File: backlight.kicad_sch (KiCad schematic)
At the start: 56 parts

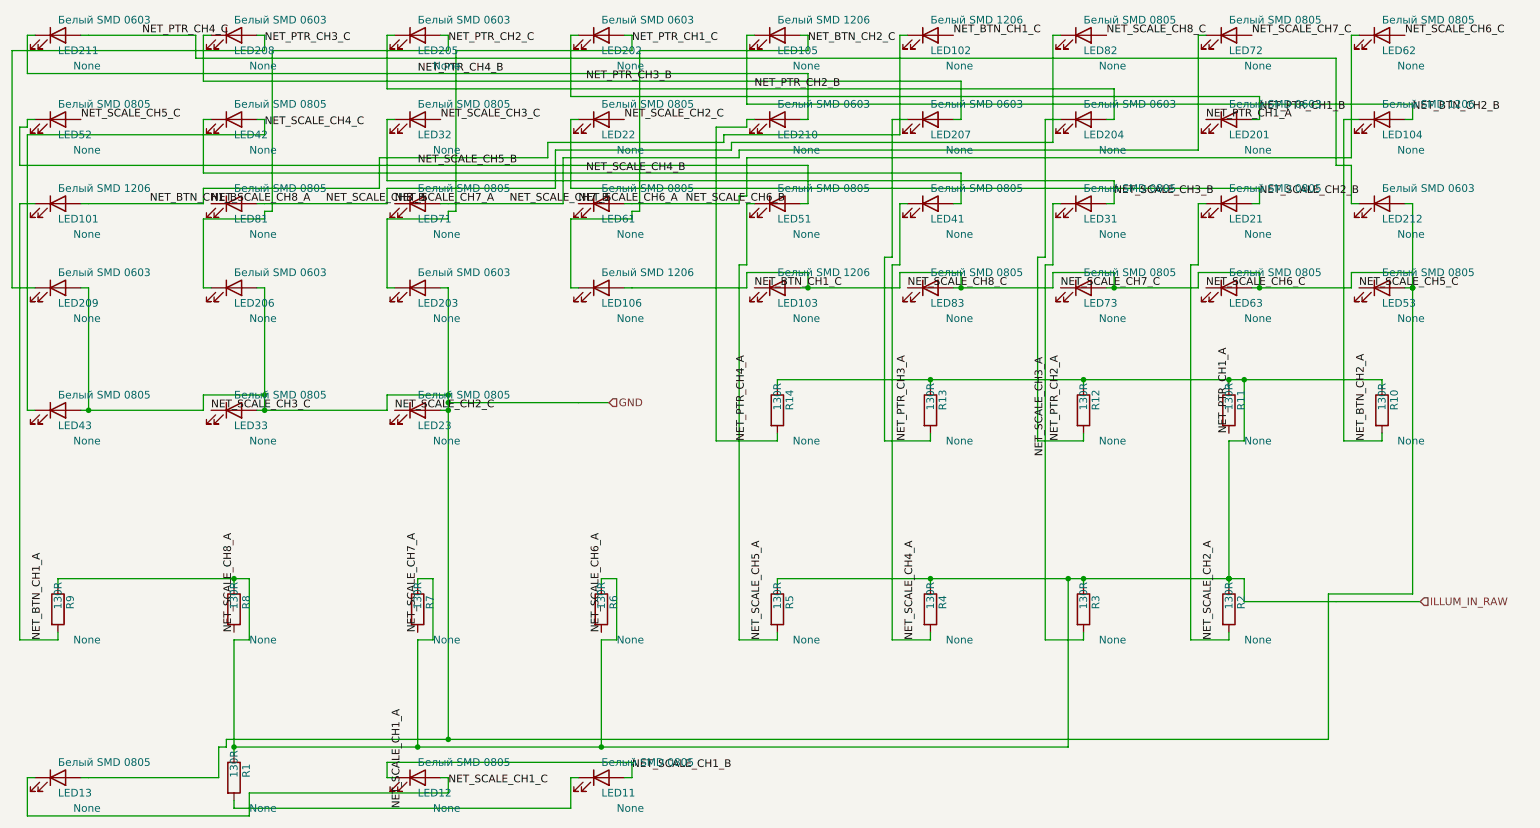
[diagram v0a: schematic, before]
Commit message: all unit test pass
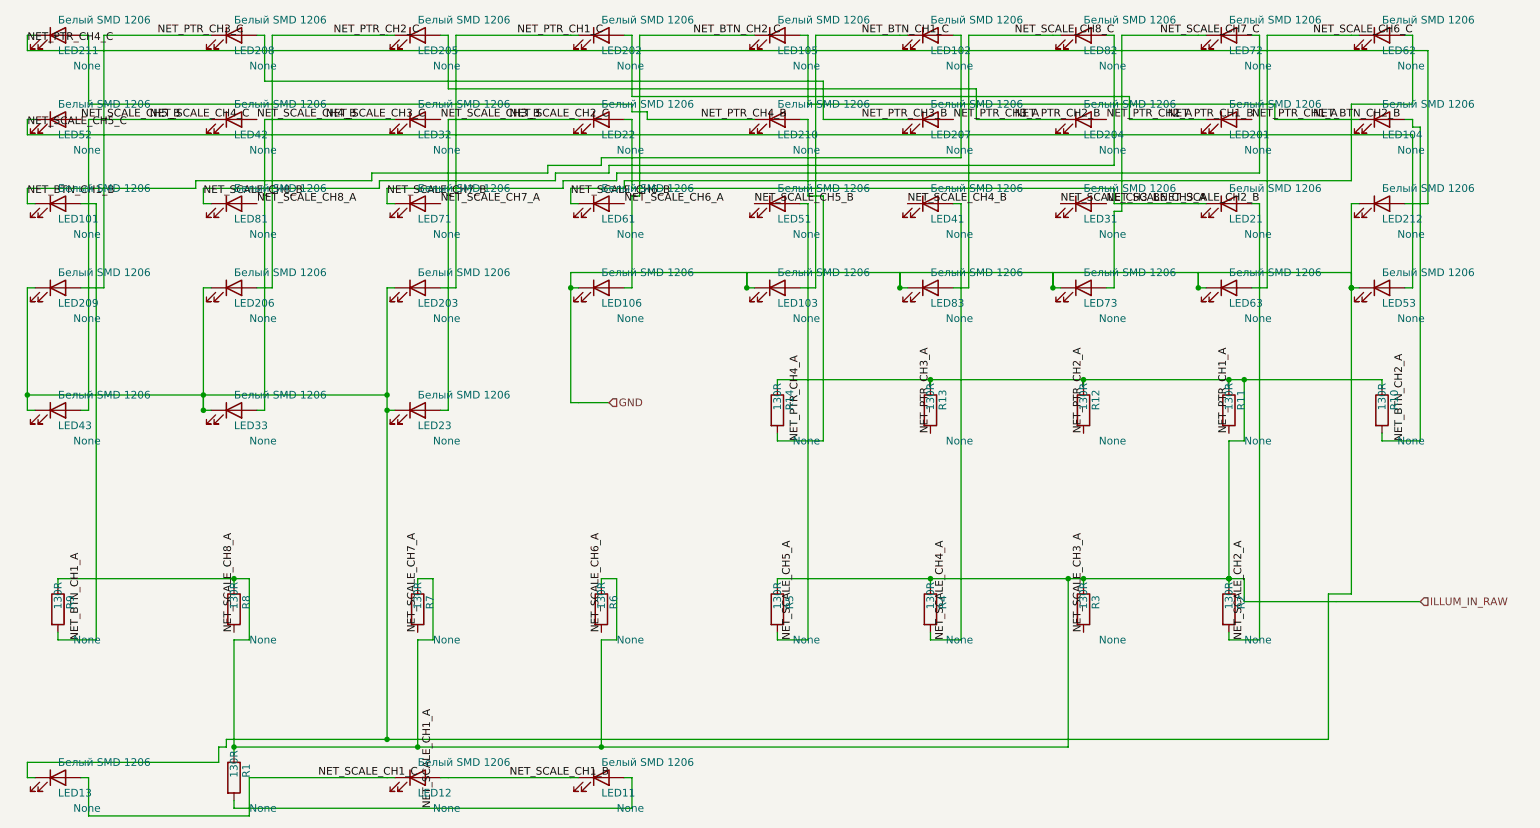
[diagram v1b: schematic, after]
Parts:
- LED11, LED12, LED13, LED21, LED22, LED23, LED31, LED32, LED33, LED41, LED42, LED43, LED51, LED52, LED53, LED61, LED62, LED63, LED71, LED72, LED73, LED81, LED82, LED83: value Белый SMD 0805 -> Белый SMD 1206
- LED201, LED202, LED203, LED204, LED205, LED206, LED207, LED208, LED209, LED210, LED211, LED212: value Белый SMD 0603 -> Белый SMD 1206
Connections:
- net GND: now also LED103.1 (K), LED106.1 (K), LED13.1 (K), LED203.1 (K), LED206.1 (K), LED209.1 (K), LED212.1 (K), LED23.1 (K), LED33.1 (K), LED43.1 (K), LED53.1 (K), LED63.1 (K), LED73.1 (K), LED83.1 (K); no longer LED103.2 (A), LED106.2 (A), LED13.2 (A), LED203.2 (A), LED206.2 (A), LED209.2 (A), LED212.2 (A), LED23.2 (A), LED33.2 (A), LED43.2 (A), LED53.2 (A), LED63.2 (A), LED73.2 (A), LED83.2 (A)
- net NET_BTN_CH1_A: now also LED101.2 (A); no longer LED101.1 (K)
- net NET_BTN_CH1_B: now also LED101.1 (K), LED102.2 (A); no longer LED101.2 (A), LED102.1 (K)
- net NET_BTN_CH1_C: now also LED102.1 (K), LED103.2 (A); no longer LED102.2 (A), LED103.1 (K)
- net NET_BTN_CH2_A: now also LED104.2 (A); no longer LED104.1 (K)
- net NET_BTN_CH2_B: now also LED104.1 (K), LED105.2 (A); no longer LED104.2 (A), LED105.1 (K)
- net NET_BTN_CH2_C: now also LED105.1 (K), LED106.2 (A); no longer LED105.2 (A), LED106.1 (K)
- net NET_PTR_CH1_A: now also LED201.2 (A); no longer LED201.1 (K)
- net NET_PTR_CH1_B: now also LED201.1 (K), LED202.2 (A); no longer LED201.2 (A), LED202.1 (K)
- net NET_PTR_CH1_C: now also LED202.1 (K), LED203.2 (A); no longer LED202.2 (A), LED203.1 (K)
- net NET_PTR_CH2_A: now also LED204.2 (A); no longer LED204.1 (K)
- net NET_PTR_CH2_B: now also LED204.1 (K), LED205.2 (A); no longer LED204.2 (A), LED205.1 (K)
- net NET_PTR_CH2_C: now also LED205.1 (K), LED206.2 (A); no longer LED205.2 (A), LED206.1 (K)
- net NET_PTR_CH3_A: now also LED207.2 (A); no longer LED207.1 (K)
- net NET_PTR_CH3_B: now also LED207.1 (K), LED208.2 (A); no longer LED207.2 (A), LED208.1 (K)
- net NET_PTR_CH3_C: now also LED208.1 (K), LED209.2 (A); no longer LED208.2 (A), LED209.1 (K)
- net NET_PTR_CH4_A: now also LED210.2 (A); no longer LED210.1 (K)
- net NET_PTR_CH4_B: now also LED210.1 (K), LED211.2 (A); no longer LED210.2 (A), LED211.1 (K)
- net NET_PTR_CH4_C: now also LED211.1 (K), LED212.2 (A); no longer LED211.2 (A), LED212.1 (K)
- net NET_SCALE_CH1_A: now also LED11.2 (A); no longer LED11.1 (K)
- net NET_SCALE_CH1_B: now also LED11.1 (K), LED12.2 (A); no longer LED11.2 (A), LED12.1 (K)
- net NET_SCALE_CH1_C: now also LED12.1 (K), LED13.2 (A); no longer LED12.2 (A), LED13.1 (K)
- net NET_SCALE_CH2_A: now also LED21.2 (A); no longer LED21.1 (K)
- net NET_SCALE_CH2_B: now also LED21.1 (K), LED22.2 (A); no longer LED21.2 (A), LED22.1 (K)
- net NET_SCALE_CH2_C: now also LED22.1 (K), LED23.2 (A); no longer LED22.2 (A), LED23.1 (K)
- net NET_SCALE_CH3_A: now also LED31.2 (A); no longer LED31.1 (K)
- net NET_SCALE_CH3_B: now also LED31.1 (K), LED32.2 (A); no longer LED31.2 (A), LED32.1 (K)
- net NET_SCALE_CH3_C: now also LED32.1 (K), LED33.2 (A); no longer LED32.2 (A), LED33.1 (K)
- net NET_SCALE_CH4_A: now also LED41.2 (A); no longer LED41.1 (K)
- net NET_SCALE_CH4_B: now also LED41.1 (K), LED42.2 (A); no longer LED41.2 (A), LED42.1 (K)
- net NET_SCALE_CH4_C: now also LED42.1 (K), LED43.2 (A); no longer LED42.2 (A), LED43.1 (K)
- net NET_SCALE_CH5_A: now also LED51.2 (A); no longer LED51.1 (K)
- net NET_SCALE_CH5_B: now also LED51.1 (K), LED52.2 (A); no longer LED51.2 (A), LED52.1 (K)
- net NET_SCALE_CH5_C: now also LED52.1 (K), LED53.2 (A); no longer LED52.2 (A), LED53.1 (K)
- net NET_SCALE_CH6_A: now also LED61.2 (A); no longer LED61.1 (K)
- net NET_SCALE_CH6_B: now also LED61.1 (K), LED62.2 (A); no longer LED61.2 (A), LED62.1 (K)
- net NET_SCALE_CH6_C: now also LED62.1 (K), LED63.2 (A); no longer LED62.2 (A), LED63.1 (K)
- net NET_SCALE_CH7_A: now also LED71.2 (A); no longer LED71.1 (K)
- net NET_SCALE_CH7_B: now also LED71.1 (K), LED72.2 (A); no longer LED71.2 (A), LED72.1 (K)
- net NET_SCALE_CH7_C: now also LED72.1 (K), LED73.2 (A); no longer LED72.2 (A), LED73.1 (K)
- net NET_SCALE_CH8_A: now also LED81.2 (A); no longer LED81.1 (K)
- net NET_SCALE_CH8_B: now also LED81.1 (K), LED82.2 (A); no longer LED81.2 (A), LED82.1 (K)
- net NET_SCALE_CH8_C: now also LED82.1 (K), LED83.2 (A); no longer LED82.2 (A), LED83.1 (K)
